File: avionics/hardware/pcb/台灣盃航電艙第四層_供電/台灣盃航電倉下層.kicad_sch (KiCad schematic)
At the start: 43 parts, among them J1 XT60, J2 XT60, J4 Pyro1, J5 Pyro2, Q1 NMOS, Q2 NMOS, Q3 NMOS, Q4 NMOS, U11 Connector, U3 LM2596S-5, U4 LM2596S-5, U5 AMS1117-3.3, U6 AMS1117-3.3

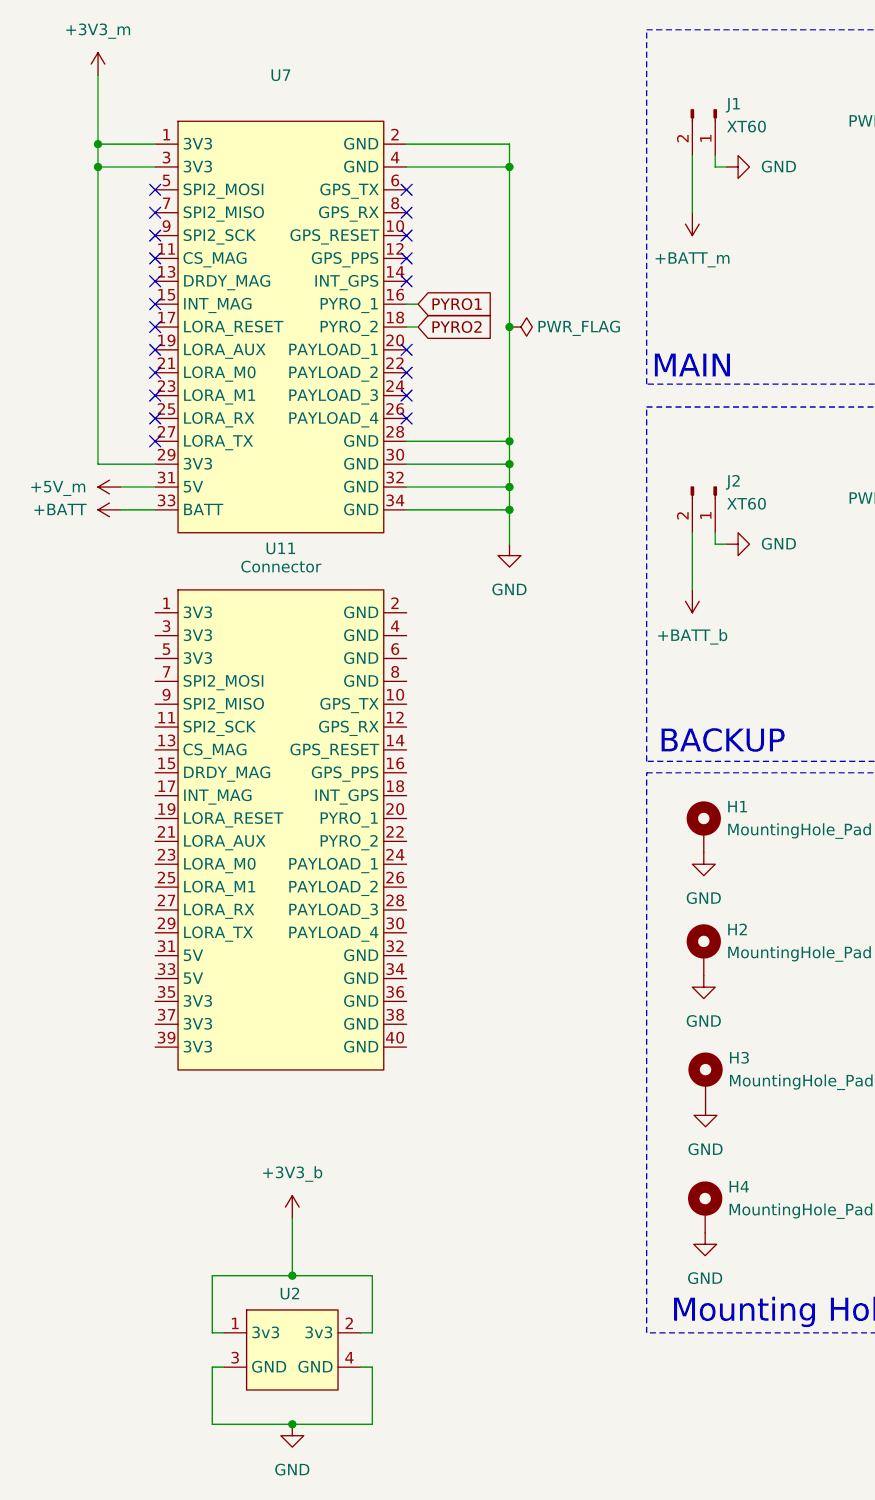
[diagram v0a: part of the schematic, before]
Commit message: Add files via upload
change schematics
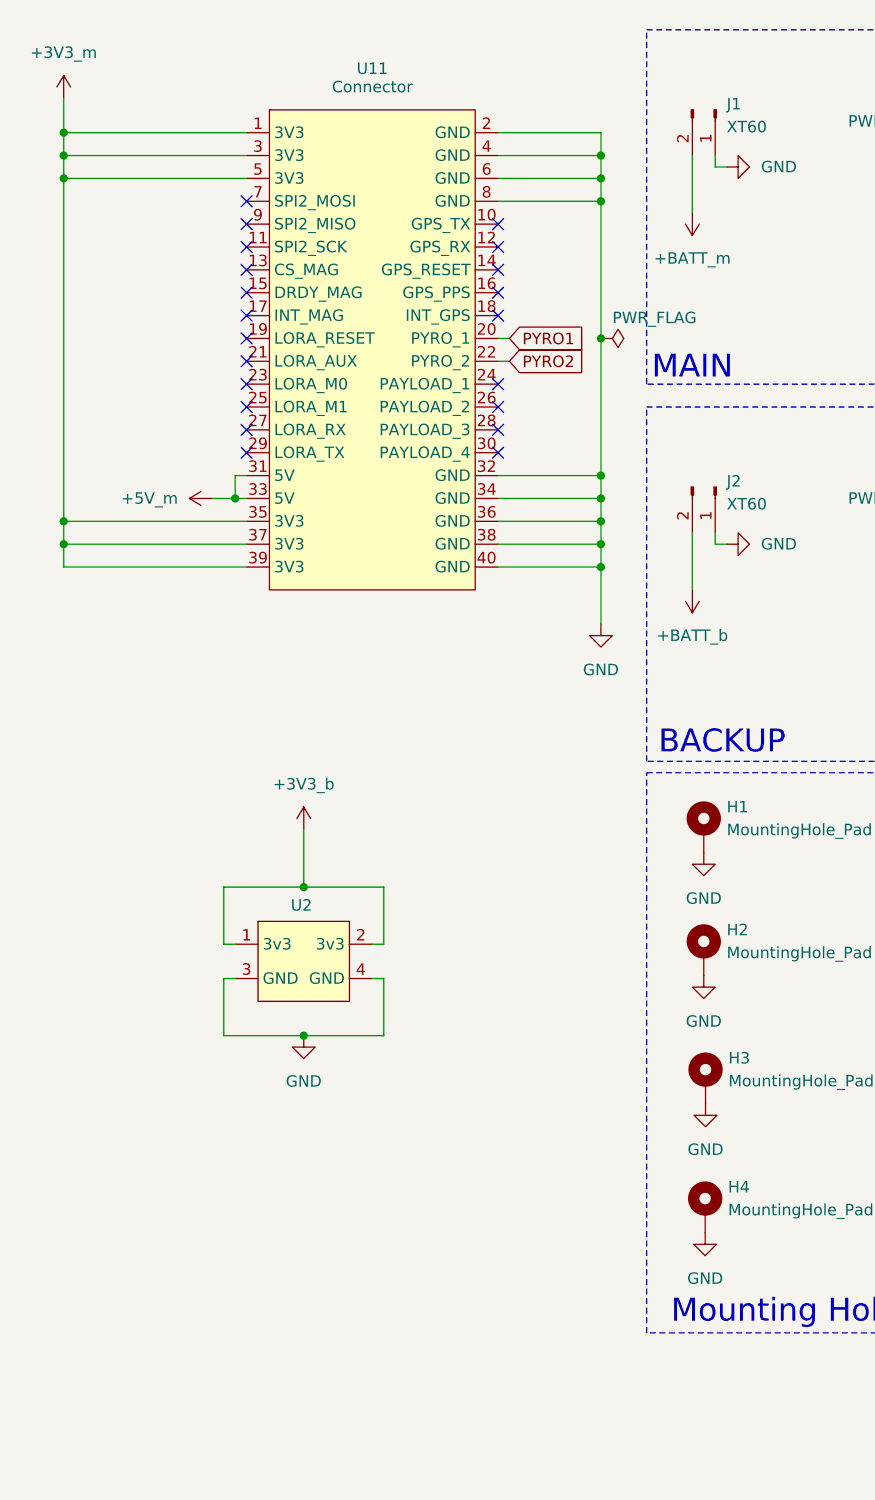
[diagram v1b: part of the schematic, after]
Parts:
- removed U7: ~, Connector_PinHeader_1.00mm:PinHeader_2x17_P1.00mm_Vertical, symbol MySymbol:2x17排針母座連接
- U11: footprint (none) -> Connector_PinHeader_2.54mm:PinHeader_2x20_P2.54mm_Vertical
- U2: footprint Connector_PinHeader_1.00mm:PinHeader_2x02_P1.00mm_Vertical -> Connector_PinHeader_2.54mm:PinHeader_2x02_P2.54mm_Vertical
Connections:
- net +3V3_m: now also U11.1 (3V3), U11.3 (3V3), U11.35 (3V3), U11.37 (3V3), U11.39 (3V3), U11.5 (3V3)
- net +5V_m: now also U11.31 (5V), U11.33 (5V)
- net GND: now also U11.2 (GND), U11.32 (GND), U11.34 (GND), U11.36 (GND), U11.38 (GND), U11.4 (GND), U11.40 (GND), U11.6 (GND), U11.8 (GND)
- net PYRO1: now also U11.20 (PYRO_1)
- net PYRO2: now also U11.22 (PYRO_2)
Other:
- moved on the sheet: U11, U2
